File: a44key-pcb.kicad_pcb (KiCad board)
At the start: 2 copper layers, 132.6 x 118.3 mm, 61 parts, among them J1 AudioJack3, SW1 SW_Push, U1 ATmega32U4-AU, Y1 16MHz

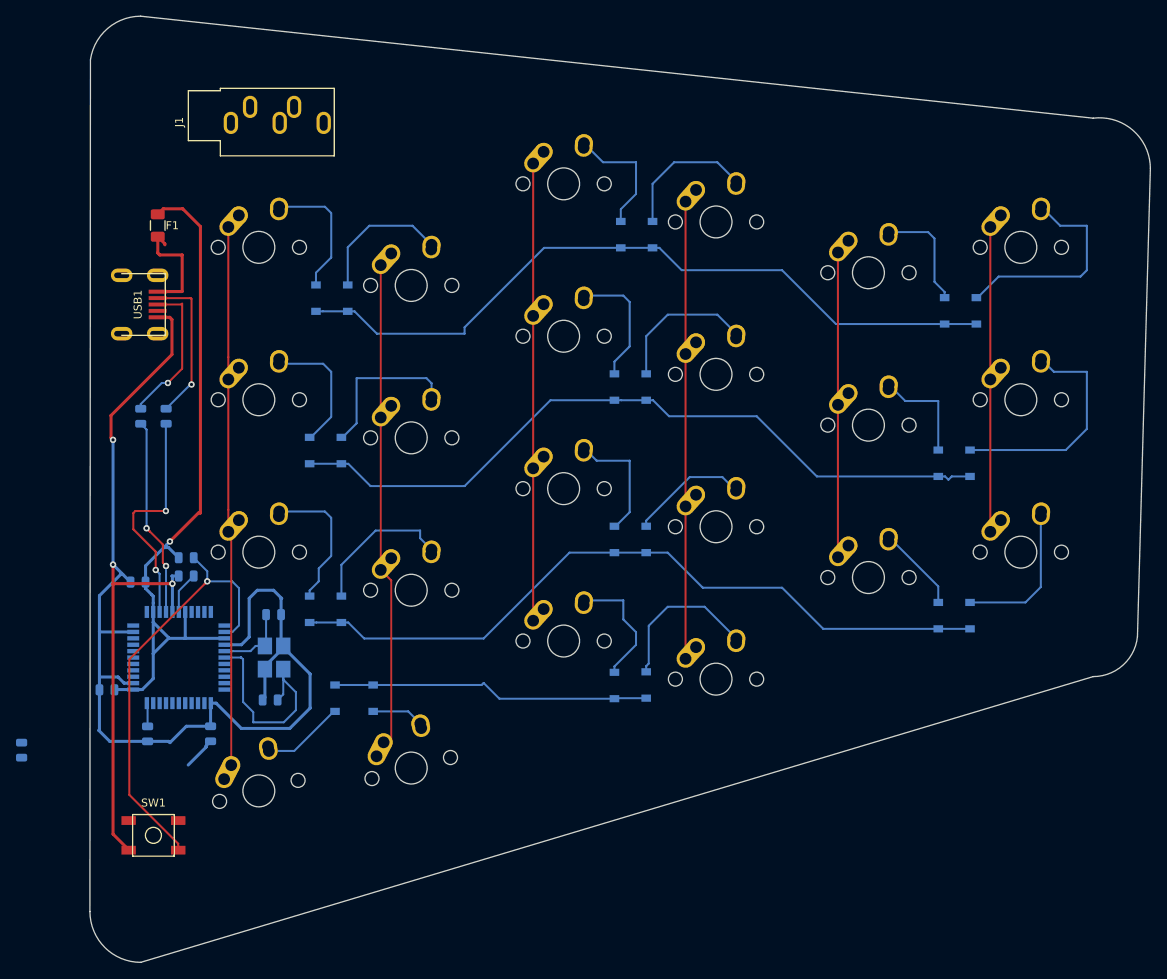
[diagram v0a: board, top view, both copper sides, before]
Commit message: Submodules added
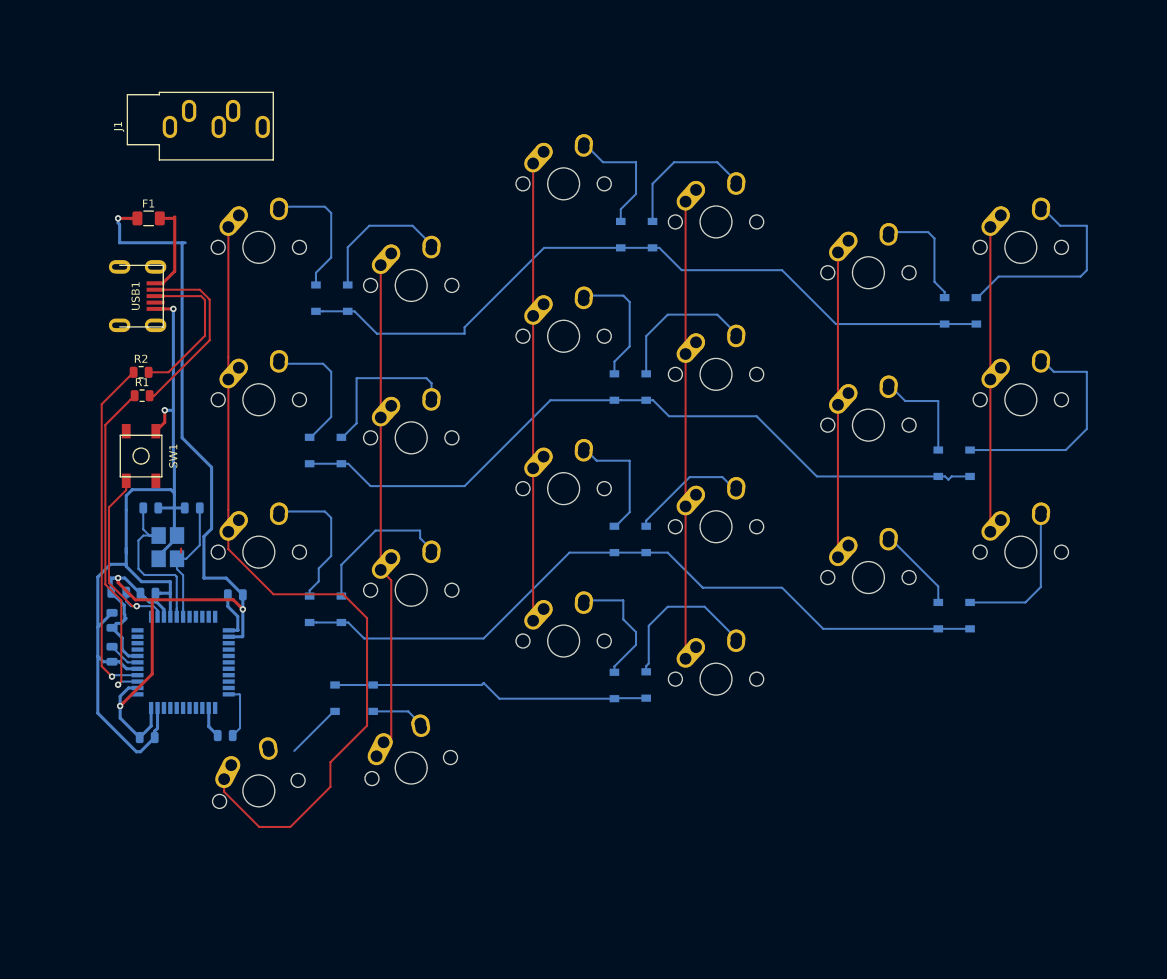
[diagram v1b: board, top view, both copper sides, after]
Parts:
- R1, R2: moved to F.Cu
- moved SW1 47.4 mm to (80.2, 96.3), turned to 90 degrees
- moved C5 33.0 mm to (92.0, 113.6), turned to 180 degrees
- moved C2 25.9 mm to (86.6, 102.7)
- moved C3 20.3 mm to (81.4, 102.7)
- moved Y1 19.2 mm to (83.6, 107.6)
- moved C6 13.5 mm to (76.6, 121.0), turned to 270 degrees
- moved R4 9.70 mm to (90.7, 131.2), turned to 0 degrees
- moved R3 9.47 mm to (77.4, 113.3)
- moved C4 8.71 mm to (76.6, 116.8), turned to 90 degrees
- moved C1 7.94 mm to (81.0, 131.4), turned to 0 degrees
- moved J1 7.64 mm to (83.8, 55.1)
- moved R2 5.49 mm to (80.2, 85.8), turned to 0 degrees
- moved R1 3.95 mm to (80.3, 88.7), turned to 0 degrees
- moved C7 1.87 mm to (81.1, 113.4), turned to 0 degrees
- moved F1 1.45 mm to (81.2, 66.5), turned to 0 degrees
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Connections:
- U1 pad 24: Net-(U1-Pad24) -> +5V
- U1 pad 44: Net-(U1-Pad24) -> +5V
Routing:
- net GND: track 187.4 -> 124.0 mm, vias 3 -> 2
- net +5V: track 94.2 -> 139.6 mm, vias 1 -> 4
- net COL5: track 69.5 -> 104.7 mm
- net Net-(R3-Pad2): track 55.0 -> 24.7 mm
- net Net-(R2-Pad1): track 25.6 -> 43.5 mm, vias 2 -> 1
- net Net-(C3-Pad1): track 9.30 -> 21.8 mm
- net Net-(R1-Pad1): track 28.8 -> 41.2 mm, vias 2 -> 1
- net Net-(C2-Pad1): track 26.7 -> 16.4 mm
- net Net-(R4-Pad2): track 2.94 -> 6.90 mm
- net Net-(D4-Pad2): track 10.3 -> 7.14 mm
- net D-: track 19.7 -> 22.7 mm, vias 1 -> 0
- net VCC: track 14.2 -> 11.7 mm
- net Net-(C6-Pad1): track 5.26 -> 4.00 mm
- net D+: track 18.8 -> 19.8 mm, vias 1 -> 0
- net (no net): track 0.00 -> 0.51 mm
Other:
- board outline removed
